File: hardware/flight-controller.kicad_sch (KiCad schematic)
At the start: 46 parts, among them J1 Screw_Terminal_01x02, U1 TPS63070RNMR, U2 ICM-45686, U3 BQ25883RGER, U4 BMP580, U5 STM32F722RETx, U6 LMR51430

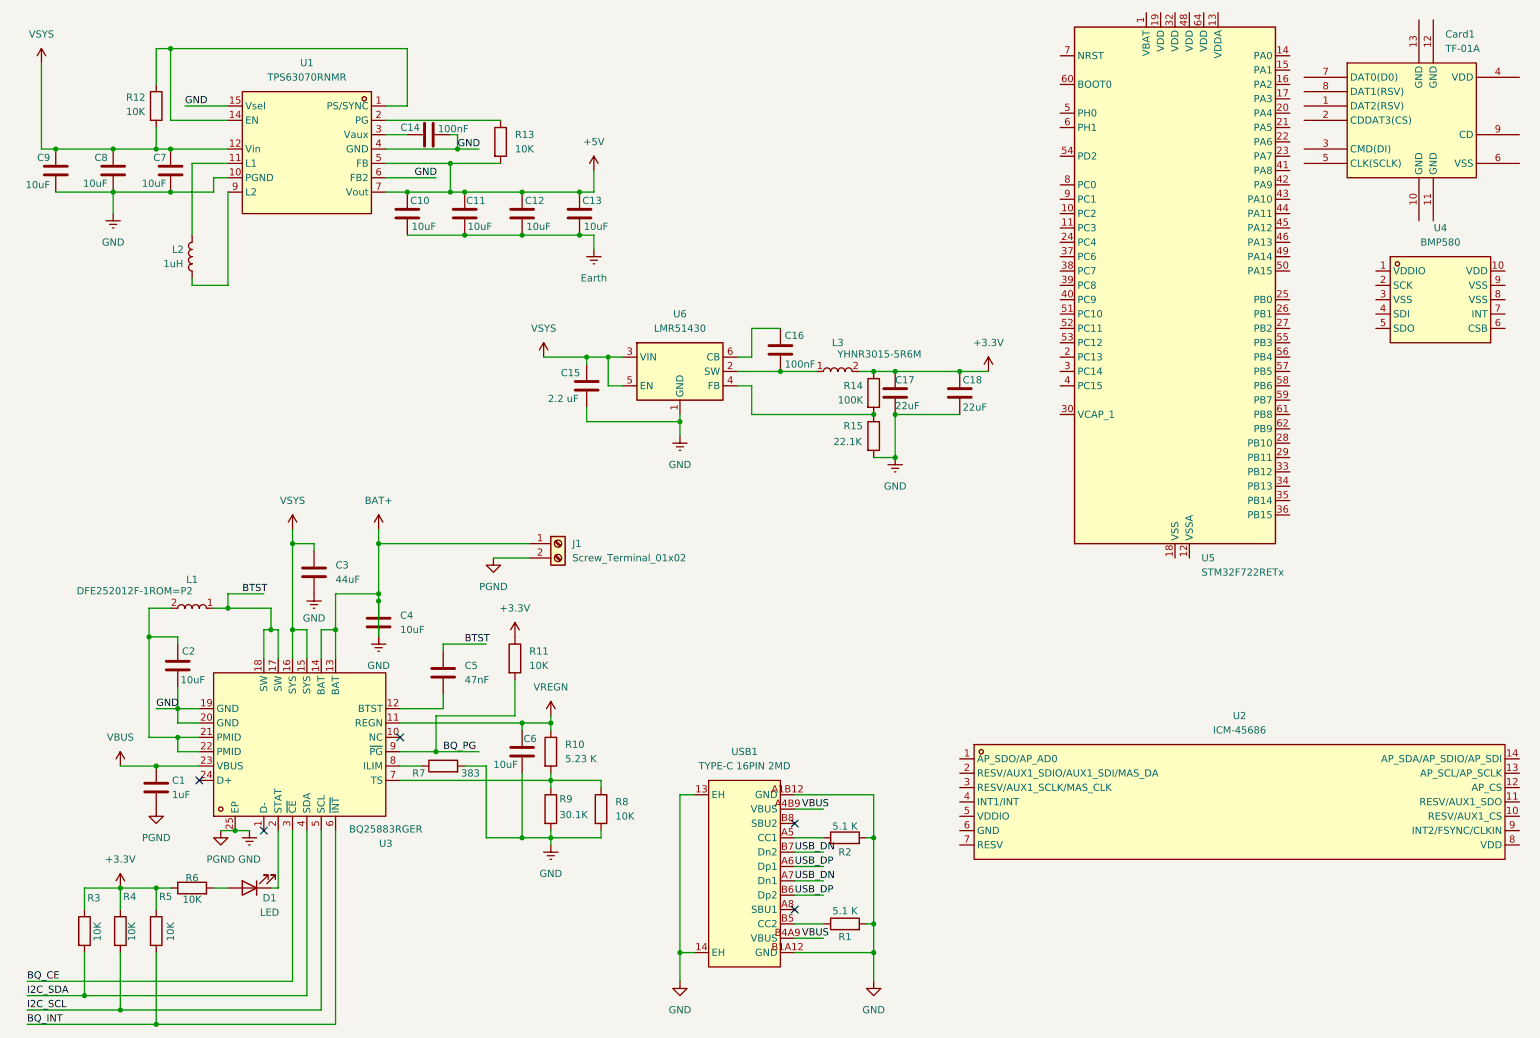
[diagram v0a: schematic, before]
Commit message: KiCad updates and journal
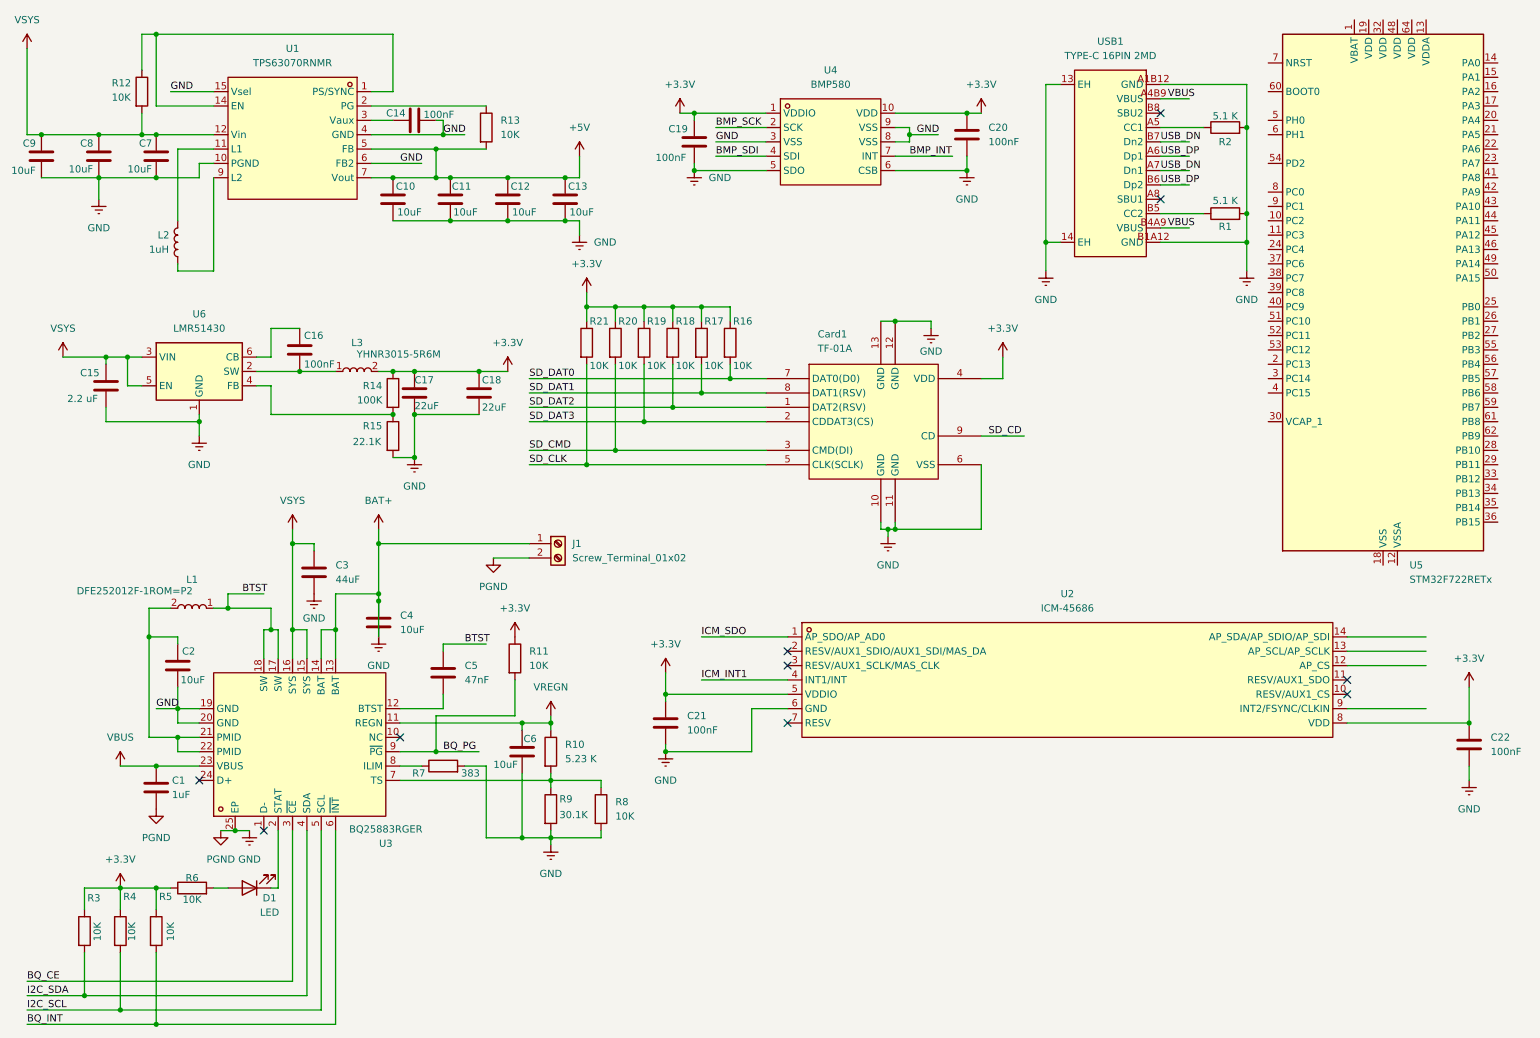
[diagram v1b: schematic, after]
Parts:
- added C19, C20, C21, C22: 100nF, symbol Device:C
- added R16, R17, R18, R19, R20, R21: 10K, symbol Device:R
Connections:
- net Earth is gone; now on net BAT+: C10.2, C11.2, C12.2, C13.2
- net +3.3V: now also Card1.4 (VDD), U2.5 (VDDIO), U2.8 (VDD), U4.1 (VDDIO), U4.10 (VDD), C19.2, C20.1, C21.1, C22.1, R16.1, R17.1, R18.1, R19.1, R20.1, R21.1
- net BAT+: now also Card1.10 (GND), Card1.11 (GND), Card1.12 (GND), Card1.13 (GND), Card1.6 (VSS), U2.6 (GND), U4.3 (VSS), U4.5 (SDO), U4.6 (CSB), U4.8 (VSS), U4.9 (VSS), C19.1, C20.2, C21.2, C22.2
- net BMP_SCK: now reaches U4.2 (SCK)
- net BMP_SDI: now reaches U4.4 (SDI)
- net BMP_INT: now reaches U4.7 (INT)
- net ICM_SDO: now reaches U2.1 (AP_SDO/AP_AD0)
- net ICM_INT1: now reaches U2.4 (INT1/INT)
- net SD_DAT2: now reaches Card1.1 (DAT2(RSV))
- net SD_DAT2: now also R18.2
- net SD_DAT3: now reaches Card1.2 (CDDAT3(CS))
- net SD_DAT3: now also R19.2
- net SD_CMD: now reaches Card1.3 (CMD(DI))
- net SD_CMD: now also R20.2
- net SD_CLK: now reaches Card1.5 (CLK(SCLK))
- net SD_CLK: now also R21.2
- net SD_DAT0: now reaches Card1.7 (DAT0(D0))
- net SD_DAT0: now also R16.2
- net SD_DAT1: now reaches Card1.8 (DAT1(RSV))
- net SD_DAT1: now also R17.2
- net SD_CD: now reaches Card1.9 (CD)
- no-connect marks 5 -> 10
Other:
- moved on the sheet: C10, C11, C12, C13, C14, C15, C16, C17, C18, C7, C8, C9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
